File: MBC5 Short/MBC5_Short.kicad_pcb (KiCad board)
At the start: 2 copper layers, 51 x 30.7 mm, 1 part, among them J1 GameBoy_GamePak_AGB-002

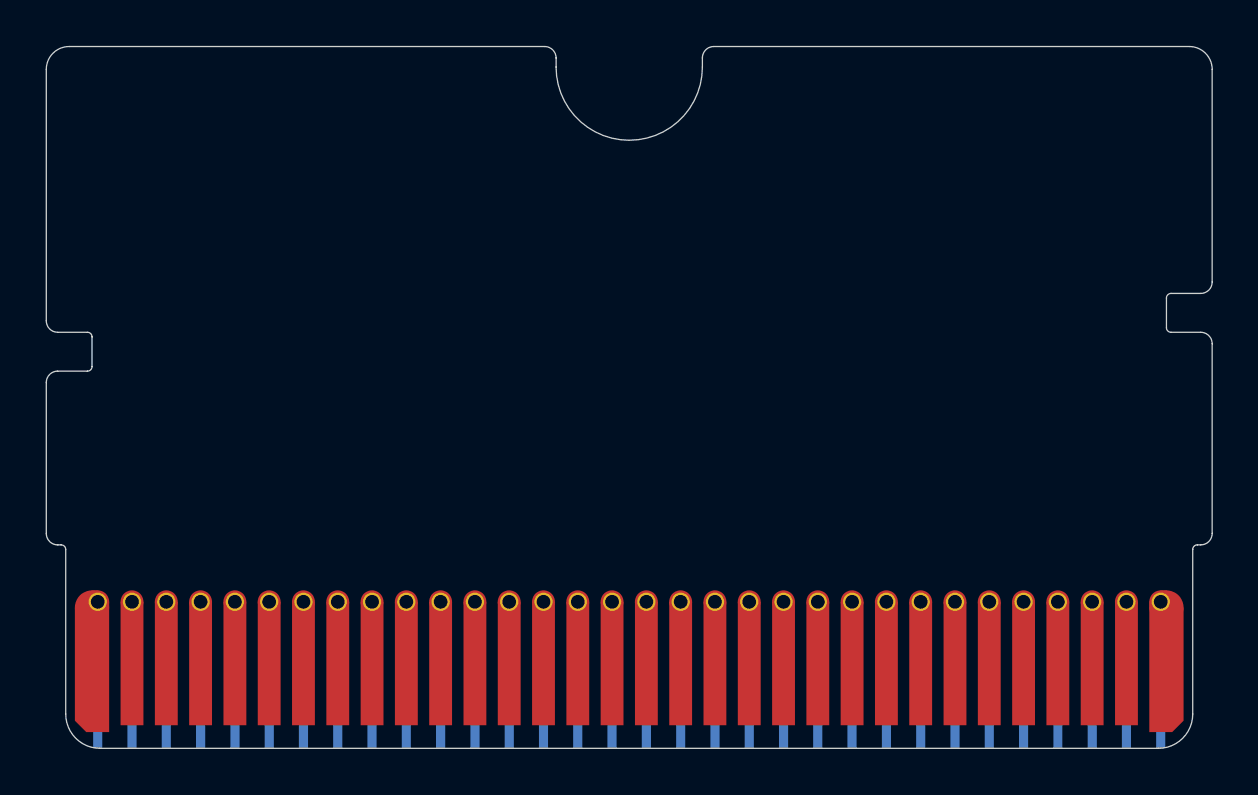
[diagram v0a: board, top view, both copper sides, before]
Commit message: Route entire board, bam
This was a lot of work, but I really didn't feel like doing micro-commits for all the changes here and there
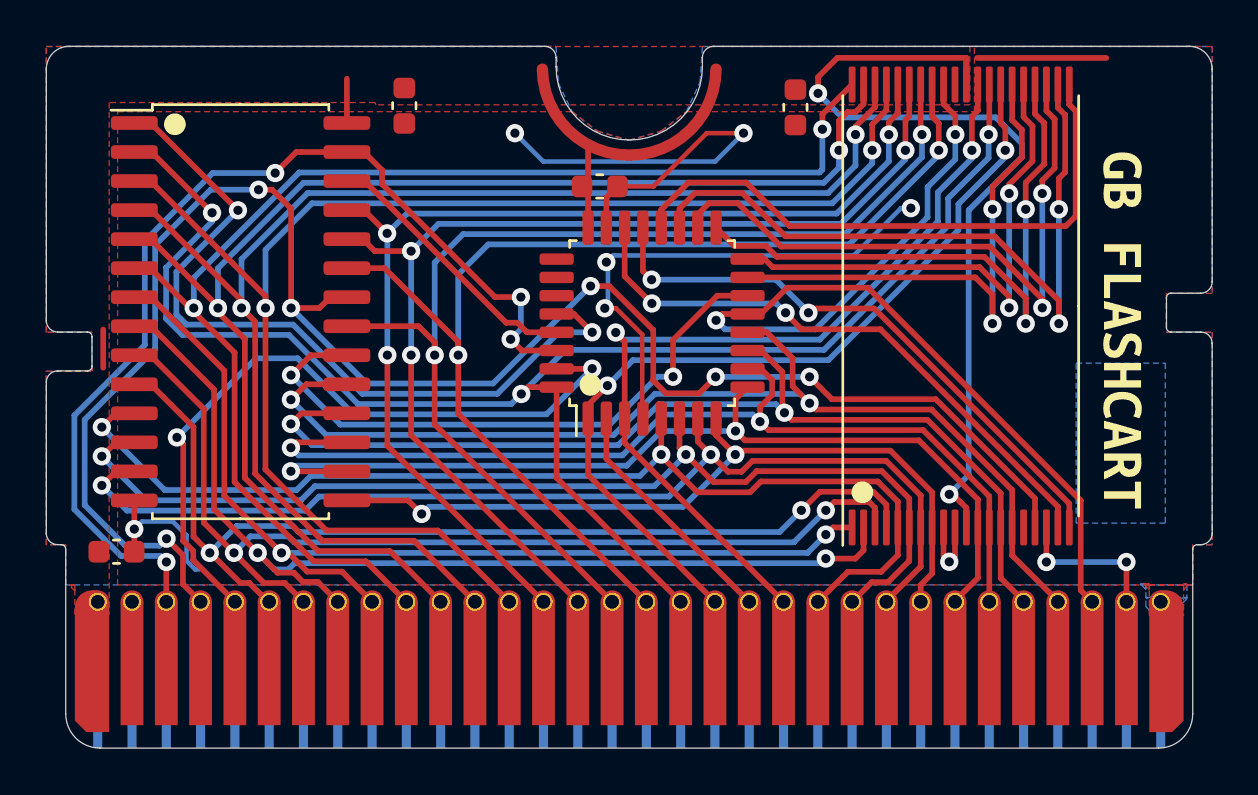
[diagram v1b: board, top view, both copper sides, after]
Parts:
- added C1: 100nF, Capacitor_SMD:C_0603_1608Metric, F.Cu at (127.6, 108.0)
- added C2: 100nF, Capacitor_SMD:C_0603_1608Metric, F.Cu at (148.7, 92.0)
- added C3: 100nF, Capacitor_SMD:C_0603_1608Metric, F.Cu at (140.2, 88.5)
- added C4: 100nF, Capacitor_SMD:C_0603_1608Metric, F.Cu at (157.3, 88.6)
- added GNDPAD: Nintendo_2.25x2.25_Fiducial, NintendoFootprints:Nintendo_2.25x2.25_Fiducial, F.Cu at (171.5, 87.8)
- added PAD*: GB-ProductionIndicator, NintendoFootprints:GB-ProductionIndicator, B.Cu at (171.6, 103.2)
- added U1: 29F033, Package_SO:TSOP-I-40_18.4x10mm_P0.5mm, F.Cu at (164.5, 97.2)
- added U2: MBC5, Package_QFP:LQFP-32_7x7mm_P0.8mm, F.Cu at (151.0, 98.0)
- added U3: FM18W08, Package_SO:SOIC-28W_7.5x17.9mm_P1.27mm, F.Cu at (133.0, 97.5)
- added kibuzzard-622AB126: G***, kibuzzard-622AB126, B.Cu at (131.4, 88.7)
- added kibuzzard-622AB1EA: G***, kibuzzard-622AB1EA, B.Cu at (138.0, 88.9)
- added kibuzzard-622CFB3C: G***, kibuzzard-622CFB3C, F.Cu at (171.5, 98.3)
- added kibuzzard-622CFB40: G***, kibuzzard-622CFB40, F.Cu at (171.6, 98.3)
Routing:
- net RD: track 0.00 -> 77.4 mm, vias 0 -> 6
- net A12: track 0.00 -> 69.2 mm, vias 0 -> 3
- net A7: track 0.00 -> 62.8 mm, vias 0 -> 2
- net A6: track 0.00 -> 60.7 mm, vias 0 -> 2
- net A5: track 0.00 -> 58.7 mm, vias 0 -> 2
- net GND: track 0.00 -> 57.6 mm, vias 0 -> 7
- net +5V: track 0.00 -> 56.7 mm, vias 0 -> 2
- net A4: track 0.00 -> 56.3 mm, vias 0 -> 2
- net A11: track 0.00 -> 50.9 mm, vias 0 -> 2
- net A10: track 0.00 -> 49.2 mm, vias 0 -> 2
- net A9: track 0.00 -> 48.0 mm, vias 0 -> 3
- net A8: track 0.00 -> 47.9 mm, vias 0 -> 3
- net D7: track 0.00 -> 47.8 mm, vias 0 -> 2
- net D0: track 0.00 -> 47.8 mm, vias 0 -> 2
- net D1: track 0.00 -> 47.5 mm, vias 0 -> 2
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- added copper zone on F.Cu, net +5V
- added copper zone on B.Cu, net GND
- added copper zone on F.Cu, net GND
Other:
- board text added: "1"
- board text added: "32"
- board text added: "GND"
- board text added: "VCC"
- board text added: "v1"
